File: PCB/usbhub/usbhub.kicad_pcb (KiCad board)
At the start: 2 copper layers, 35 parts, among them U1 SL2.1S, U2 SL2.1S

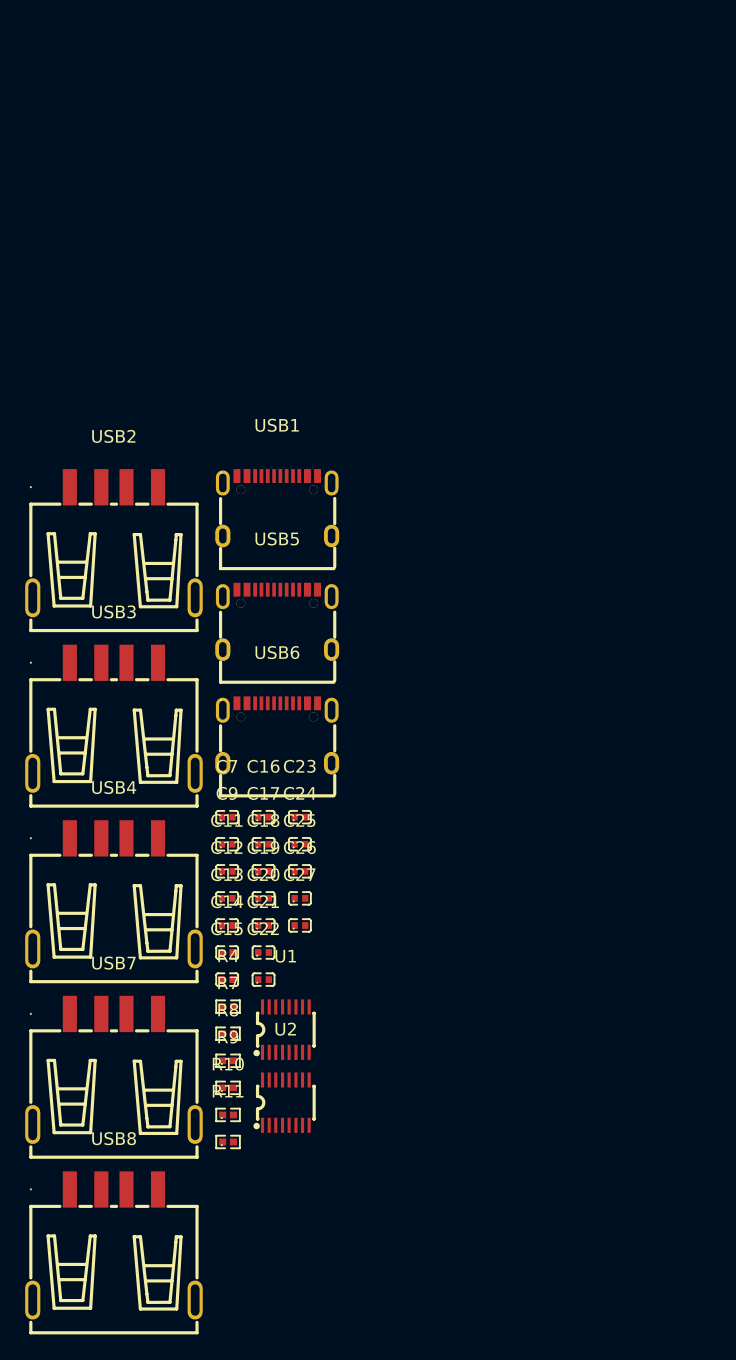
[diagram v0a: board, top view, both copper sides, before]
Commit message: placement
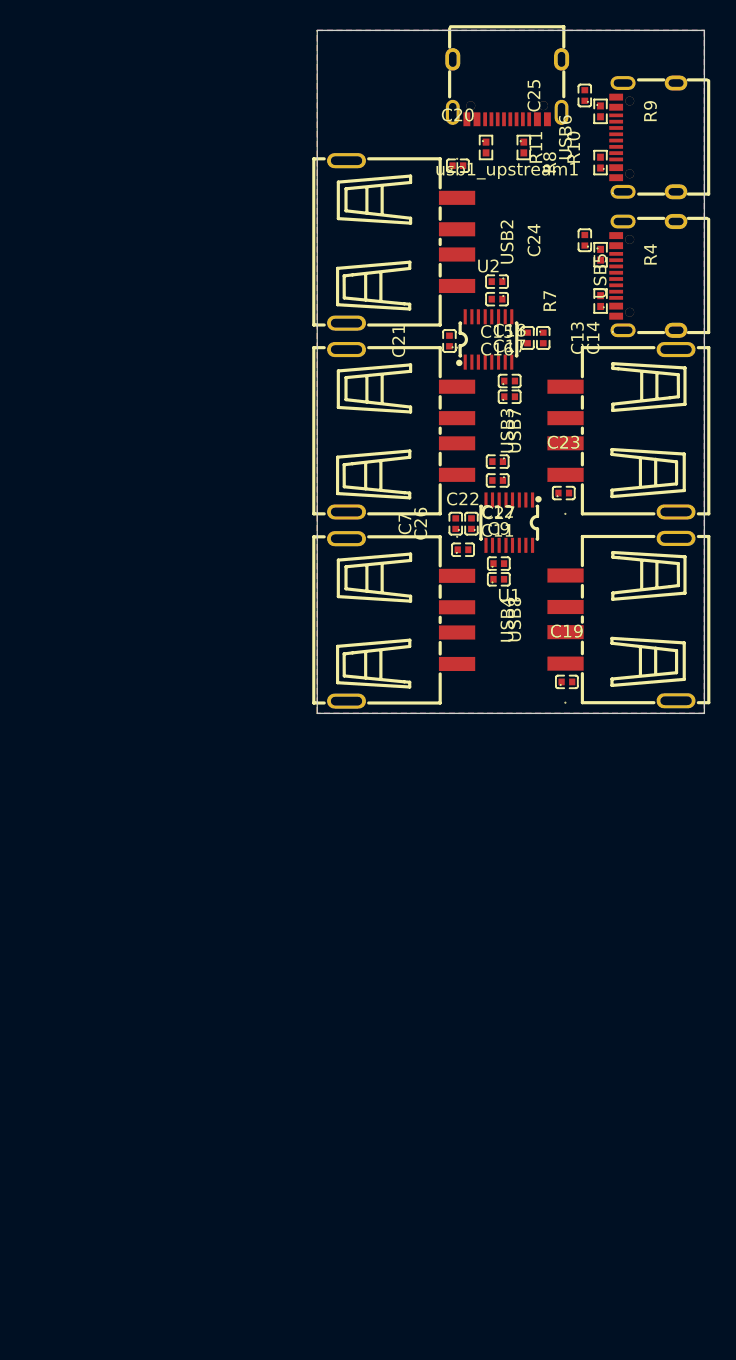
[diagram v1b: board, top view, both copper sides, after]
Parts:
- moved R9 83.0 mm to (171.0, 48.2), turned to -90 degrees
- moved R11 81.6 mm to (161.9, 51.0), turned to -90 degrees
- moved R10 80.4 mm to (164.9, 51.0), turned to -90 degrees
- moved R8 77.2 mm to (171.0, 52.2), turned to 90 degrees
- moved R4 66.7 mm to (171.0, 59.6), turned to -90 degrees
- moved C25 65.6 mm to (169.8, 46.9), turned to 90 degrees
- moved R7 65.3 mm to (171.0, 63.2), turned to 90 degrees
- moved USB7 64.8 mm to (172.6, 73.5), turned to 90 degrees
- moved USB8 63.9 mm to (172.6, 88.5), turned to 90 degrees
- moved U2 62.7 mm to (162.1, 66.3)
- moved C20 62.3 mm to (159.7, 52.5)
- moved C15 59.4 mm to (162.8, 61.7), turned to 180 degrees
- moved USB6 55.7 mm to (174.6, 50.2), turned to 90 degrees
- moved C14 54.9 mm to (166.4, 66.2), turned to -90 degrees
- moved C24 53.0 mm to (169.8, 58.4), turned to 90 degrees
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- renumbered USB1 to usb1_upstream1
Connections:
- net /DN1A renamed /D1A-
- net /DN1B renamed /D1B-
- net /DN2A renamed /D2A-
- net /DN2B renamed /D2B-
- net /DN3A renamed /D3A-
- net /DN3B renamed /D3B-
- net /DN4B renamed /D4B-
- net /DNA renamed /DA-
- net /DNB renamed /DB-
- net /DP1A renamed /D1A+
- net /DP1B renamed /D1B+
- net /DP2A renamed /D2A+
- net /DP2B renamed /D2B+
- net /DP3A renamed /D3A+
- net /DP3B renamed /D3B+
- net /DP4B renamed /D4B+
- net /DPA renamed /DA+
- net /DPB renamed /DB+
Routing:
- added copper zone on B.Cu, net GND
- added copper zone on F.Cu, net GND
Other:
- board outline added: 30.8 x 54.2 mm
